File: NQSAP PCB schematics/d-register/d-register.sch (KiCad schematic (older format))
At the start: 52 parts, among them J1 Bus, J2 Bus, J5 Conn_01x04, J6 Conn_01x08, U1 74HCT377, U2 74HCT245, U3 74LS283, U4 74LS283, U5 74HCT138, U6 74HCT138

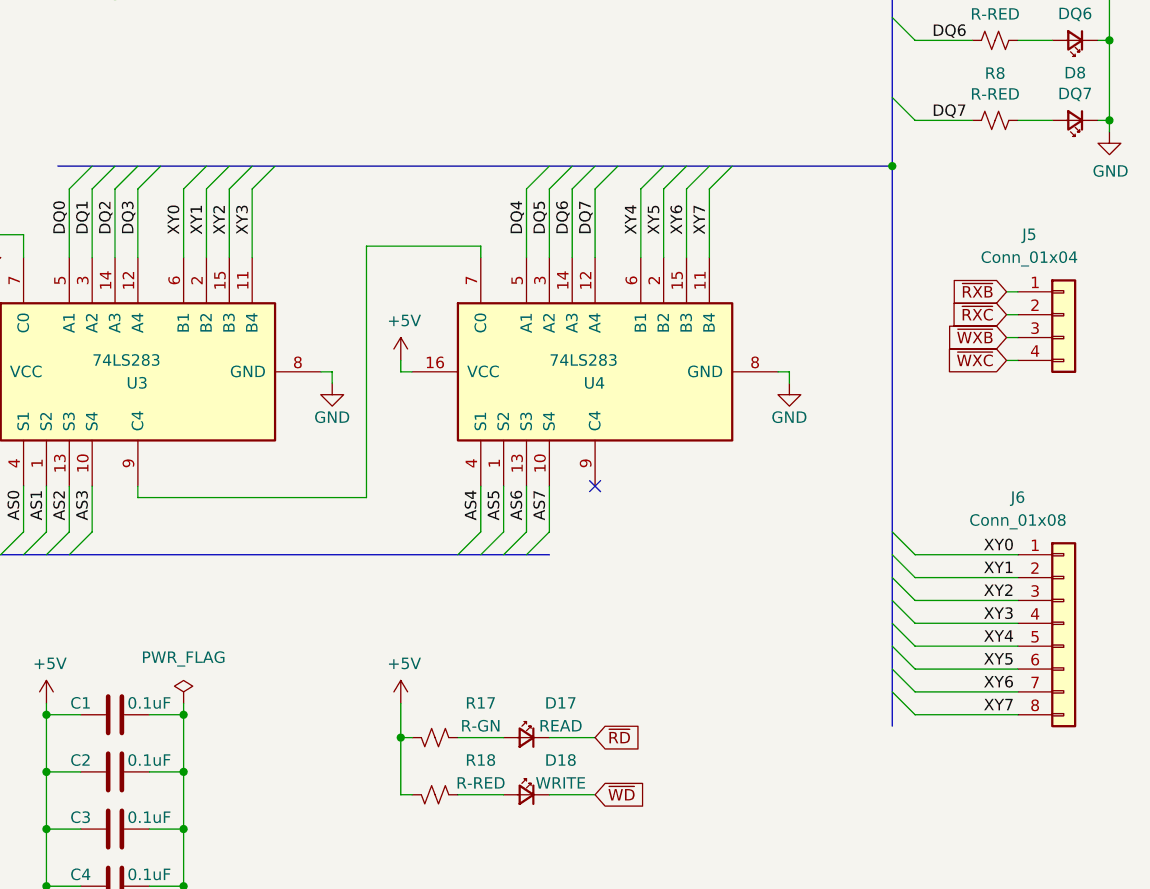
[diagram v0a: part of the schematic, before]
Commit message: build 5 board updates
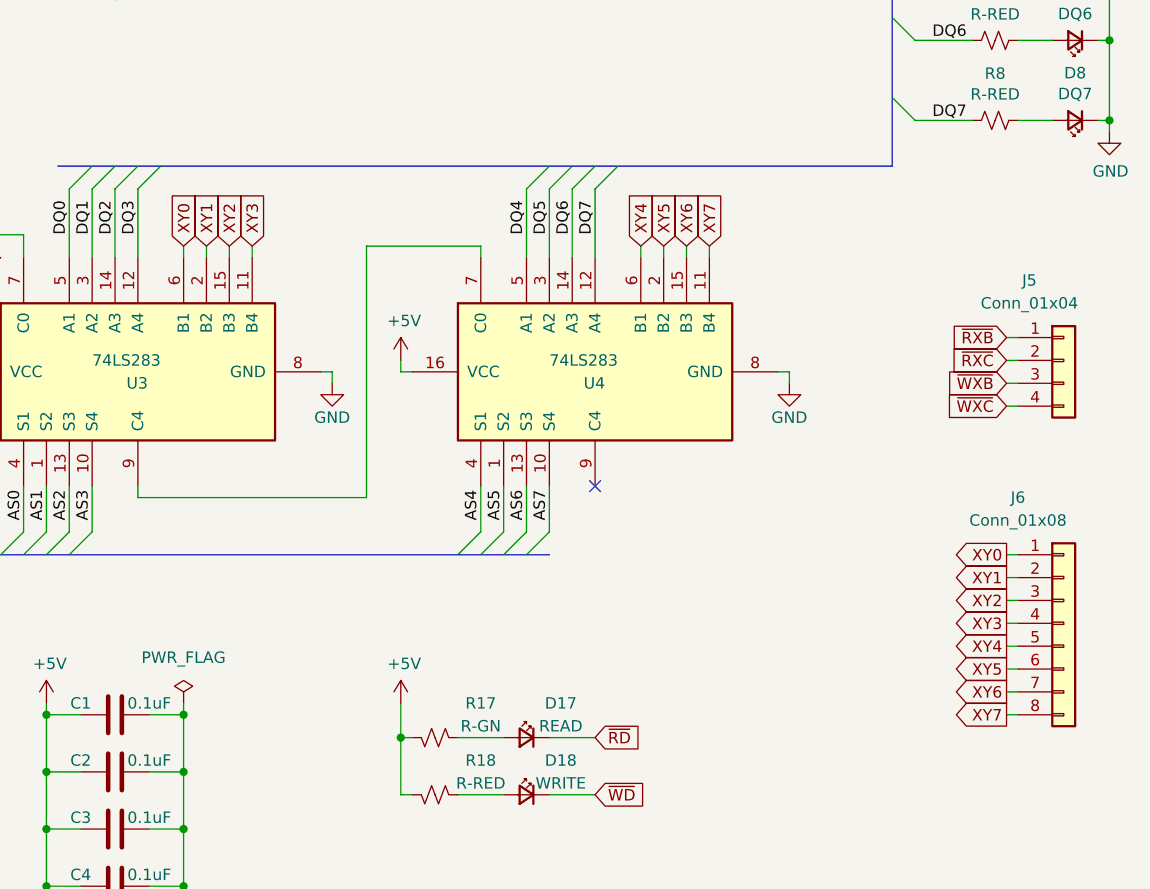
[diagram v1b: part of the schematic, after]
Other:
- moved on the sheet: J5
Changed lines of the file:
@@
 L Connector_Generic:Conn_01x04 J5
 U 1 1 6167BE3C
-P 9550 4300
-F 0 "J5" H 9400 4650 50  0000 C CNN
-F 1 "Conn_01x04" H 9400 4550 50  0000 C CNN
-F 2 "Connector_PinHeader_2.54mm:PinHeader_1x04_P2.54mm_Vertical" H 9550 4300 50  0001 C CNN
-F 3 "~" H 9550 4300 50  0001 C CNN
-	1    9550 4300
+P 9550 4500
+F 0 "J5" H 9400 4850 50  0000 C CNN
+F 1 "Conn_01x04" H 9400 4750 50  0000 C CNN
+F 2 "Connector_PinHeader_2.54mm:PinHeader_1x04_P2.54mm_Vertical" H 9550 4500 50  0001 C CNN
+F 3 "~" H 9550 4500 50  0001 C CNN
+	1    9550 4500
 	1    0    0    -1
 $EndComp
@@
 Text Label 6050 1400 2    50   ~ 0
 D7
-Entry Wire Line
-	8800 5250 8900 5350
-Wire Wire Line
-	8900 5350 9350 5350
-Entry Wire Line
-	8800 5350 8900 5450
-Wire Wire Line
-	8900 5450 9350 5450
-Entry Wire Line
-	8800 5450 8900 5550
-Wire Wire Line
-	8900 5550 9350 5550
-Entry Wire Line
-	8800 5550 8900 5650
-Wire Wire Line
-	8900 5650 9350 5650
-Entry Wire Line
-	8800 5650 8900 5750
-Wire Wire Line
-	8900 5750 9350 5750
-Entry Wire Line
-	8800 5750 8900 5850
-Wire Wire Line
-	8900 5850 9350 5850
-Entry Wire Line
-	8800 5850 8900 5950
-Wire Wire Line
-	8900 5950 9350 5950
-Entry Wire Line
-	8800 5950 8900 6050
-Wire Wire Line
-	8900 6050 9350 6050
-Text Label 9200 5350 0    50   ~ 0
-XY0
-Text Label 9200 5450 0    50   ~ 0
-XY1
-Text Label 9200 5550 0    50   ~ 0
-XY2
-Text Label 9200 5650 0    50   ~ 0
-XY3
-Text Label 9200 5750 0    50   ~ 0
-XY4
-Text Label 9200 5850 0    50   ~ 0
-XY5
-Text Label 9200 5950 0    50   ~ 0
-XY6
-Text Label 9200 6050 0    50   ~ 0
-XY7
+Wire Wire Line
+	5700 4000 5700 4050
 Text GLabel 1050 6850 0    50   Input ~ 0
 WR3
@@
 Wire Wire Line
 	4400 6650 4300 6650
-Text GLabel 9300 4500 0    50   Input ~ 0
+Text GLabel 9300 4700 0    50   Input ~ 0
 ~WXC
 Text GLabel 4800 2400 0    50   Input ~ 0
 ~RD
-Text GLabel 9300 4300 0    50   Input ~ 0
+Text GLabel 9300 4500 0    50   Input ~ 0
 ~RXC
-Text GLabel 9300 4200 0    50   Input ~ 0
+Text GLabel 9300 4400 0    50   Input ~ 0
 ~RXB
 Wire Wire Line
@@
 Wire Wire Line
 	2150 6650 2250 6650
-Text GLabel 9300 4400 0    50   Input ~ 0
+Text GLabel 9300 4600 0    50   Input ~ 0
 ~WXB
 NoConn ~ 1050 4700
@@
 Wire Wire Line
 	6650 6150 6650 6400
-Connection ~ 8800 3650
 Connection ~ 5100 6300
 Connection ~ 5700 6300
@@
 	5200 4050 5200 3750
 Entry Wire Line
-	6100 3650 6000 3750
-Wire Wire Line
-	6000 4050 6000 3750
-Entry Wire Line
-	6000 3650 5900 3750
-Wire Wire Line
-	5900 4050 5900 3750
-Entry Wire Line
-	5900 3650 5800 3750
-Wire Wire Line
-	5800 4050 5800 3750
-Entry Wire Line
-	5800 3650 5700 3750
-Wire Wire Line
-	5700 4050 5700 3750
-Entry Wire Line
 	7600 3650 7500 3750
 Wire Wire Line
@@
 Wire Wire Line
 	7200 4050 7200 3750
-Entry Wire Line
-	8100 3650 8000 3750
-Wire Wire Line
-	8000 4050 8000 3750
-Entry Wire Line
-	8000 3650 7900 3750
-Wire Wire Line
-	7900 4050 7900 3750
-Entry Wire Line
-	7900 3650 7800 3750
-Wire Wire Line
-	7800 4050 7800 3750
-Entry Wire Line
-	7800 3650 7700 3750
-Wire Wire Line
-	7700 4050 7700 3750
 Text Label 5000 5200 1    50   ~ 0
 AS0
@@
 NoConn ~ 2250 7050
 Wire Wire Line
-	9350 4200 9300 4200
-Wire Wire Line
-	9350 4300 9300 4300
-Wire Wire Line
 	9350 4400 9300 4400
 Wire Wire Line
 	9350 4500 9300 4500
+Wire Wire Line
+	9350 4600 9300 4600
+Wire Wire Line
+	9350 4700 9300 4700
 $Comp
 L power:+5V #PWR0117
@@
 Text Label 7500 3950 1    50   ~ 0
 DQ7
-Text Label 5700 3950 1    50   ~ 0
+NoConn ~ 1050 4400
+Text GLabel 5700 4000 1    50   Input ~ 0
 XY0
-Text Label 5800 3950 1    50   ~ 0
+Wire Wire Line
+	5800 4000 5800 4050
+Text GLabel 5800 4000 1    50   Input ~ 0
 XY1
-Text Label 5900 3950 1    50   ~ 0
+Wire Wire Line
+	5900 4000 5900 4050
+Text GLabel 5900 4000 1    50   Input ~ 0
 XY2
-Text Label 6000 3950 1    50   ~ 0
+Wire Wire Line
+	6000 4000 6000 4050
+Text GLabel 6000 4000 1    50   Input ~ 0
 XY3
-Text Label 7700 3950 1    50   ~ 0
+Wire Wire Line
+	9300 5750 9350 5750
+Wire Wire Line
+	9300 5850 9350 5850
+Wire Wire Line
+	9300 5950 9350 5950
+Wire Wire Line
+	9300 6050 9350 6050
+Text GLabel 9300 6050 0    50   Output ~ 0
+XY7
+Text GLabel 9300 5950 0    50   Output ~ 0
+XY6
+Text GLabel 9300 5850 0    50   Output ~ 0
+XY5
+Text GLabel 9300 5750 0    50   Output ~ 0
 XY4
-Text Label 7800 3950 1    50   ~ 0
+Text GLabel 8000 4000 1    50   Input ~ 0
+XY7
+Text GLabel 7900 4000 1    50   Input ~ 0
+XY6
+Text GLabel 7800 4000 1    50   Input ~ 0
 XY5
-Text Label 7900 3950 1    50   ~ 0
-XY6
-Text Label 8000 3950 1    50   ~ 0
-XY7
-NoConn ~ 1050 4400
-Wire Bus Line
-	8800 3650 8800 6100
+Text GLabel 7700 4000 1    50   Input ~ 0
+XY4
+Wire Wire Line
+	7700 4000 7700 4050
+Wire Wire Line
+	7800 4000 7800 4050
+Wire Wire Line
+	7900 4000 7900 4050
+Wire Wire Line
+	8000 4000 8000 4050
+Wire Wire Line
+	9300 5350 9350 5350
+Wire Wire Line
+	9300 5450 9350 5450
+Wire Wire Line
+	9300 5550 9350 5550
+Wire Wire Line
+	9300 5650 9350 5650
+Text GLabel 9300 5650 0    50   Output ~ 0
+XY3
+Text GLabel 9300 5550 0    50   Output ~ 0
+XY2
+Text GLabel 9300 5450 0    50   Output ~ 0
+XY1
+Text GLabel 9300 5350 0    50   Output ~ 0
+XY0
 Wire Bus Line
 	4300 5350 7300 5350
@@
 	8800 750  8800 3650
 Wire Bus Line
+	5150 3650 8800 3650
+Wire Bus Line
 	4300 1250 4300 5350
-Wire Bus Line
-	5150 3650 8800 3650
 $EndSCHEMATC
